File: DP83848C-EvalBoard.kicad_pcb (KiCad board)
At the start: 4 copper layers, 75 x 100 mm, 180 parts, among them J1 Conn_01x02, J10 Conn_02x04_Odd_Even, J11 Conn_02x04_Odd_Even, J12 Conn_02x04_Odd_Even, J13 Conn_02x04_Odd_Even, J14 Conn_02x04_Odd_Even, J2 RJ45_LED_Shielded, J3 USB_C_Receptacle_USB2.0, J4 Conn_02x05_Odd_Even, J5 Conn_01x04, J6 Conn_01x04, J7 Conn_01x04, J8 Conn_02x08_Odd_Even, J9 Conn_02x08_Odd_Even, Q1 AO3401A, Q2 AO3400A, Q3 AO3401A, SW1 SW_Push, T1 H1102NL, U1 AMS1117-3.3, U10 CM1224, U11 CM1224, U12 CM1224, U13 CM1224, U14 CM1224, U15 CM1224, U2 DP83848C, U3 STM32F407VGTx, U4 USBLC6-2SC6, U5 CM1224, U6 CM1224, U7 CM1224, U8 CM1224, U9 CM1224, X1 50MHz, Y1 25MHz

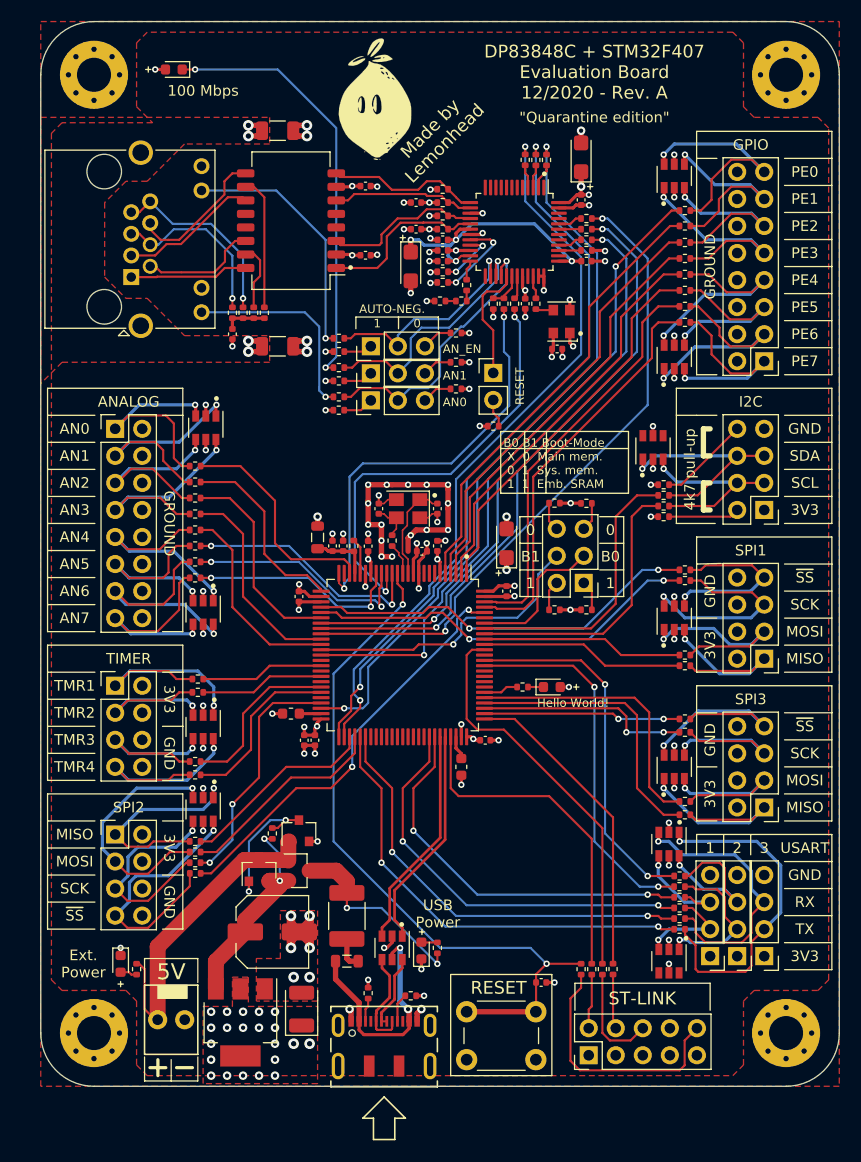
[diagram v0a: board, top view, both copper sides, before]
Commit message: Text
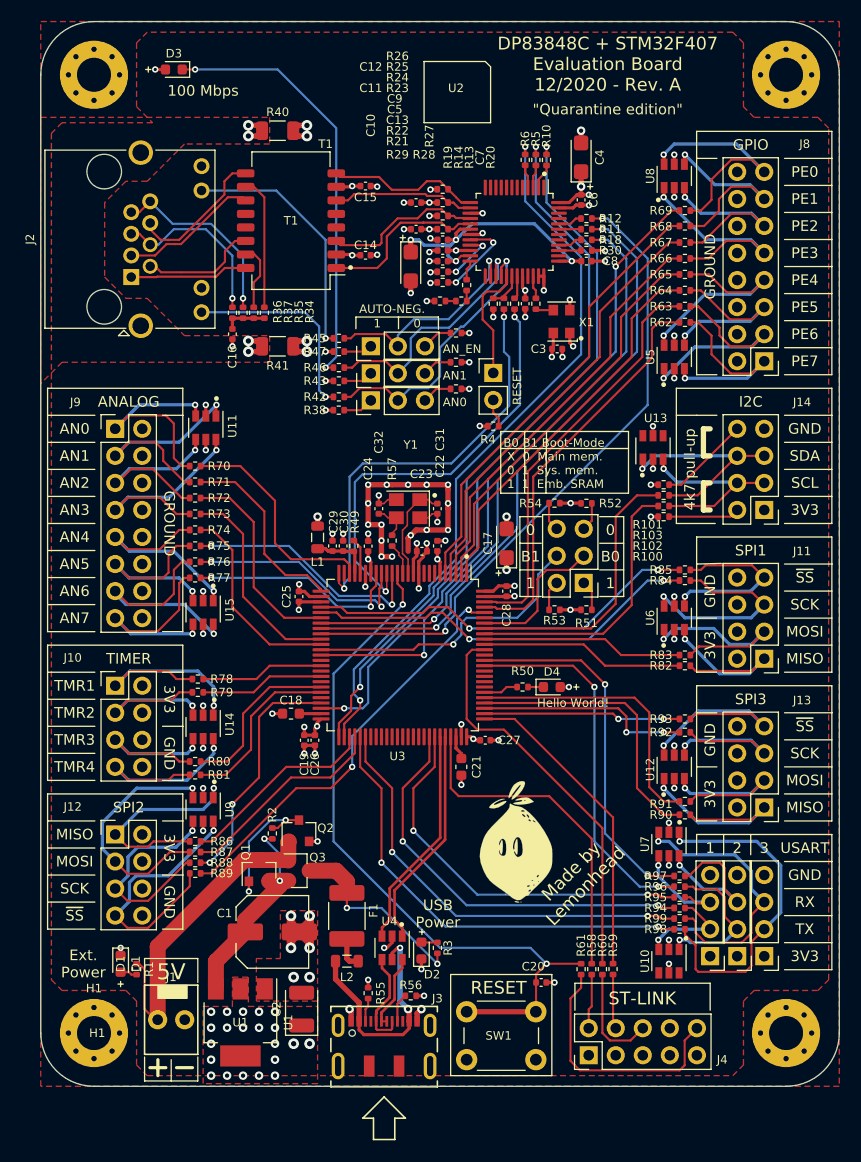
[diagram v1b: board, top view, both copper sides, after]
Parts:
- C31, C32: value TBD -> 18pF
- D3: value YL -> YE
- R100, R101: value 4k7 -> 4.7k
- R49: value 0R -> 0
- Y1: value 25MHz -> 25MHz, 10ppm, 12pF
- moved G*** 71.0 mm to (84.8, 133.8)

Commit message: Revert "Text"
This reverts commit 08ad5a624c52bb92dd714530982a715c3c379f2a.
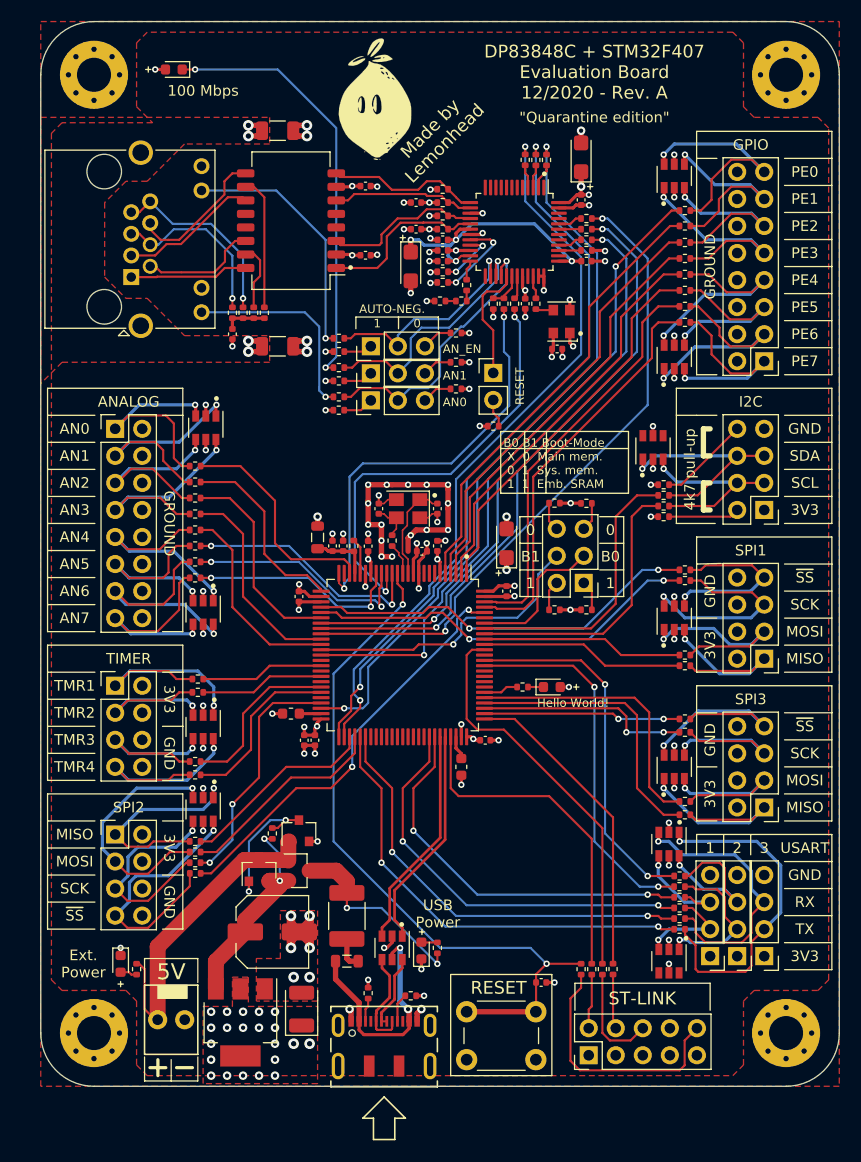
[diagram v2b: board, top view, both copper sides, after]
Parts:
- C31, C32: value 18pF -> TBD
- D3: value YE -> YL
- R100, R101: value 4.7k -> 4k7
- R49: value 0 -> 0R
- Y1: value 25MHz, 10ppm, 12pF -> 25MHz
- moved G*** 71.0 mm to (71.5, 64.0)
